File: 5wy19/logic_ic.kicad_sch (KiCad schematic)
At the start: 25 parts, among them IC9 0504TAK, Q14 BAW56, Q23 BZX84Cxx, Q25 BC846, Q27 BCR183, Q28 BCR183, U2 74HC32, U4 74HC08

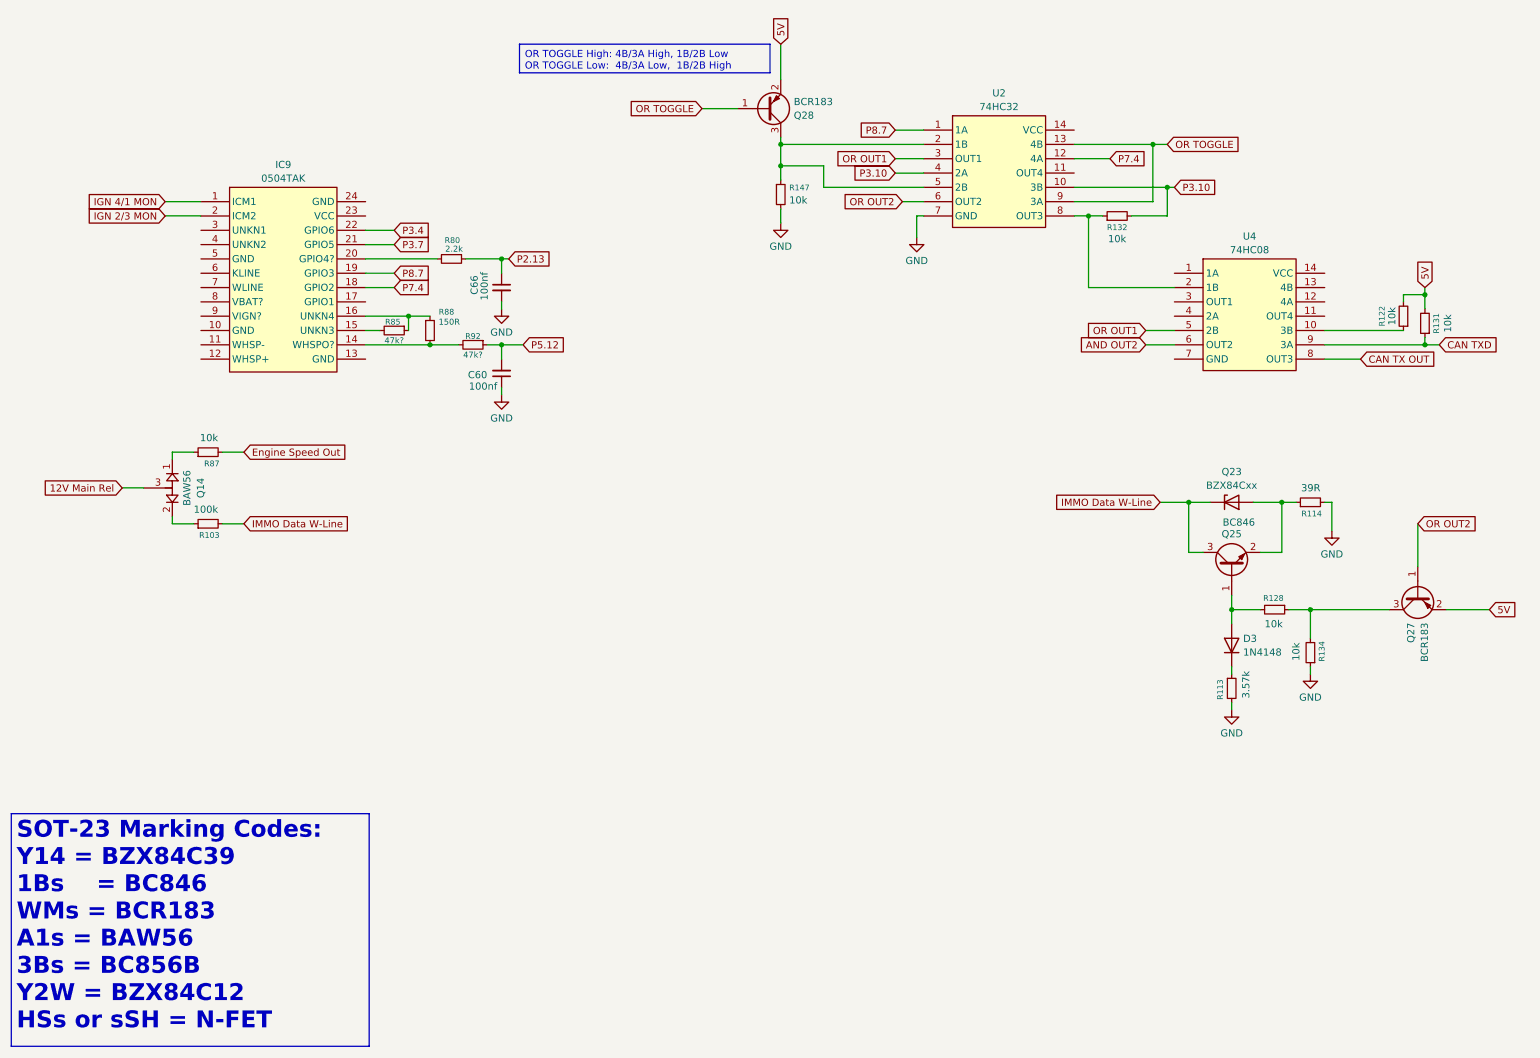
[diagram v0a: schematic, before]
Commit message: Final schematic (except maybe some oversights)
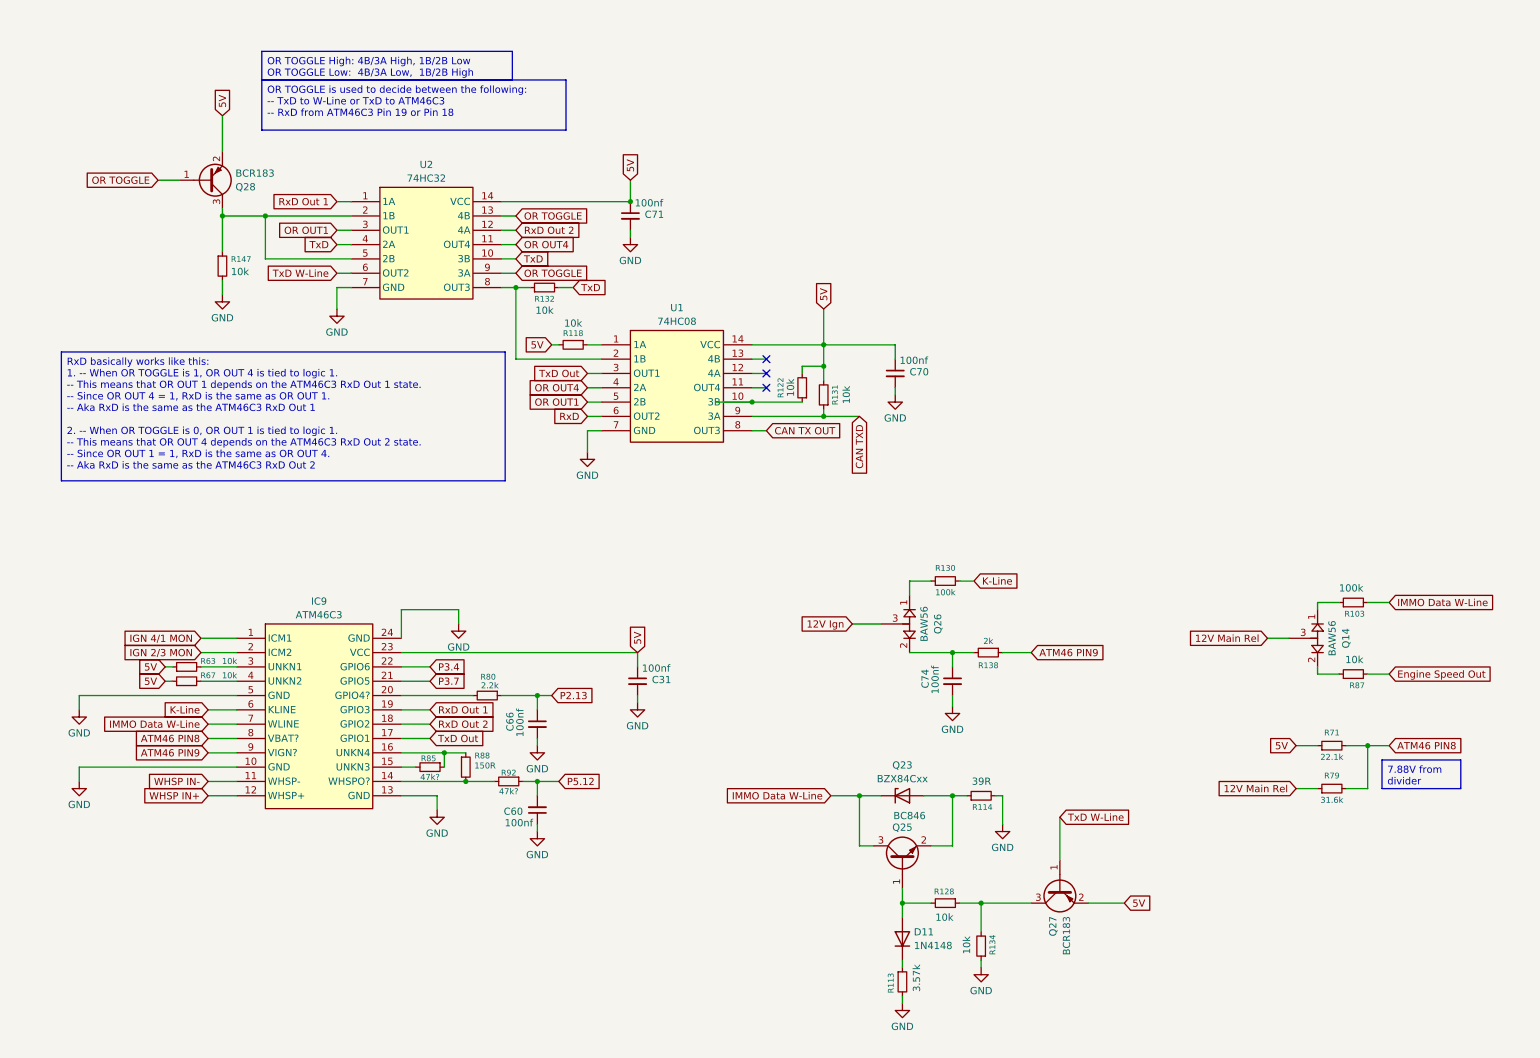
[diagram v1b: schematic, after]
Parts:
- added C31, C70, C71, C74: 100nf, symbol Device:C_Small
- added Q26: BAW56, symbol SIMK43:BAW56
- added R118, R63, R67: 10k, symbol Device:R_Small
- added R130: 100k, symbol Device:R_Small
- added R138: 2k, symbol Device:R_Small
- added R71: 22.1k, symbol Device:R_Small
- added R79: 31.6k, symbol Device:R_Small
- IC9: value 0504TAK -> ATM46C3
- renumbered D3 to D11, U4 to U1
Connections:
- net 12V Main Rel: now also R79.1
- net 5V: now also IC9.23 (VCC), U1.14 (VCC), U2.14 (VCC), C31.1, C70.1, C71.1, R118.2, R63.1, R67.1, R71.1
- net GND: now also IC9.10 (GND), IC9.13 (GND), IC9.24 (GND), IC9.5 (GND), U1.7 (GND), C31.2, C70.2, C71.2, C74.2
- net IMMO Data W-Line: now also IC9.7 (WLINE)
- net at R87.1: now also Q14.2; no longer Q14.1
- net at R103.1: now also Q14.1; no longer Q14.2
- net WHSP IN-: now reaches IC9.11 (WHSP-)
- net WHSP IN+: now reaches IC9.12 (WHSP+)
- net TxD Out: now reaches IC9.17 (GPIO1)
- net TxD Out: now also U1.3 (OUT1)
- net at IC9.3 (UNKN1): now also R63.2
- net at IC9.4 (UNKN2): now also R67.2
- net K-Line: now reaches IC9.6 (KLINE)
- net K-Line: now also R130.2
- net ATM46 PIN8: now reaches IC9.8 (VBAT?)
- net ATM46 PIN8: now also R71.2, R79.2
- net ATM46 PIN9: now reaches IC9.9 (VIGN?)
- net ATM46 PIN9: now also R138.1
- net OR OUT4: now reaches U2.11 (OUT4)
- net OR OUT4: now also U1.4 (2A)
- net at U1.1 (1A): now also R118.1
- net AND OUT2 renamed RxD
- net OR OUT2 renamed TxD W-Line
- net P3.10 renamed TxD
- net P7.4 renamed RxD Out 2
- net P8.7 renamed RxD Out 1
- new net: C74.1, Q26.2, R138.2
- new net: Q26.1, R130.1
- new net 12V Ign: Q26.3
- no-connect marks 0 -> 3
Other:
- moved on the sheet: C60, C66, D11, IC9, Q14, Q23, Q25, Q27, Q28, R103, R113, R114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
